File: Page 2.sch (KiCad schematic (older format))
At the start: 17 parts, among them J201 Battery Connector, Q201 BSS138, U201 MIC5219-5.0YM5-TR, U202 MIC5219-3.3YM5-TR

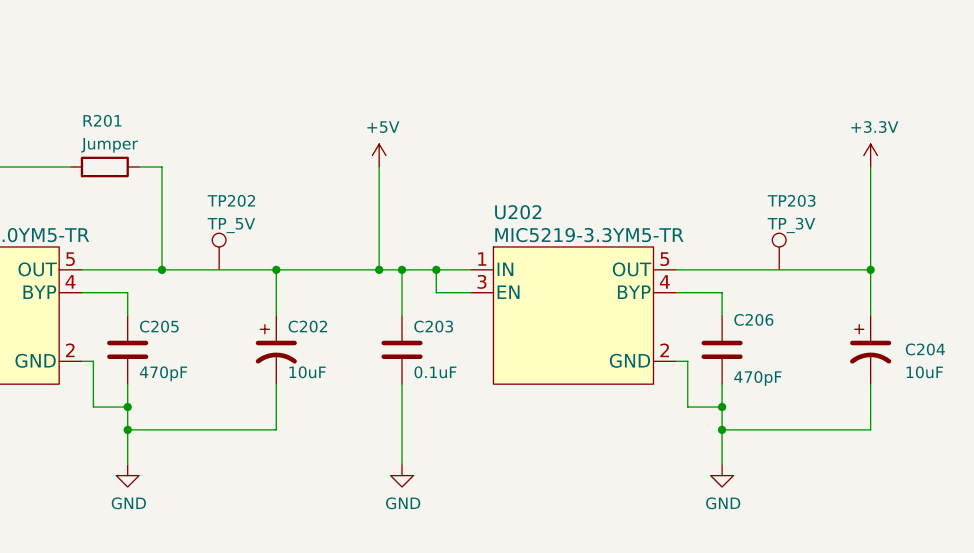
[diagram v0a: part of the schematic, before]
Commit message: PCB Update
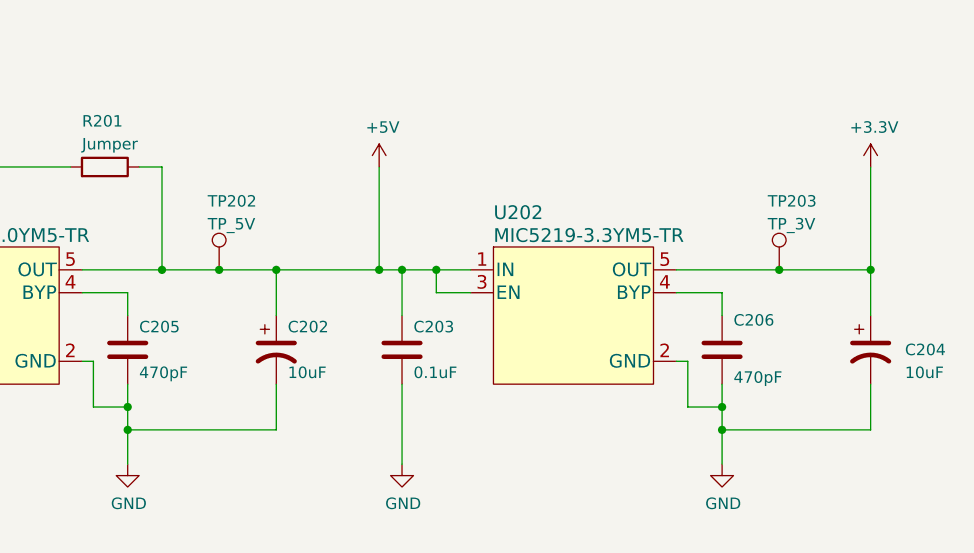
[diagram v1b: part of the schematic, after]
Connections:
- net +3V3: now also TP203.1
- net +5V: now also TP202.1
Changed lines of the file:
@@
 	4500 4050 5200 4050
 Wire Wire Line
-	8850 3500 9700 3500
+	8850 3500 9300 3500
 Wire Wire Line
-	6600 3500 7100 3500
+	6600 3500 6850 3500
 Text Label 1600 3500 0    50   ~ 0
 B+
@@
 Wire Wire Line
 	5200 4050 5300 4050
+Connection ~ 6850 3500
+Wire Wire Line
+	6850 3500 7100 3500
+Connection ~ 9300 3500
+Wire Wire Line
+	9300 3500 9700 3500
 $EndSCHEMATC

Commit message: Updates
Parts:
- U201, U202: footprint Package_TO_SOT_SMD:SOT-23-5_HandSoldering -> Package_TO_SOT_SMD:SOT-23-5
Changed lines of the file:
@@
 F 0 "U202" H 8050 4150 60  0000 L CNN
 F 1 "MIC5219-3.3YM5-TR" H 8050 4050 60  0000 L CNN
-F 2 "Package_TO_SOT_SMD:SOT-23-5_HandSoldering" H 8050 3300 60  0001 L CNN
+F 2 "Package_TO_SOT_SMD:SOT-23-5" H 8050 3300 60  0001 L CNN
 F 3 "http://ww1.microchip.com/downloads/en/DeviceDoc/MIC5219-500mA-Peak-Output-LDO-Regulator-DS20006021A.pdf" H 7750 3900 60  0001 C CNN
 F 4 "576-1281-6-ND" H 8400 3700 50  0001 C CNN "DigiKey Part No."
@@
 F 0 "U201" H 5450 4150 60  0000 L CNN
 F 1 "MIC5219-5.0YM5-TR" H 5450 4050 60  0000 L CNN
-F 2 "Package_TO_SOT_SMD:SOT-23-5_HandSoldering" H 5450 3300 60  0001 L CNN
+F 2 "Package_TO_SOT_SMD:SOT-23-5" H 5450 3300 60  0001 L CNN
 F 3 "http://ww1.microchip.com/downloads/en/DeviceDoc/MIC5219-500mA-Peak-Output-LDO-Regulator-DS20006021A.pdf" H 5150 3900 60  0001 C CNN
 F 4 "576-2770-6-ND" H 5800 3700 50  0001 C CNN "DigiKey Part No."
